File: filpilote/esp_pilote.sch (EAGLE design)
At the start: 22 parts, among them IC1 ACS758LCB-050B-PFF-T

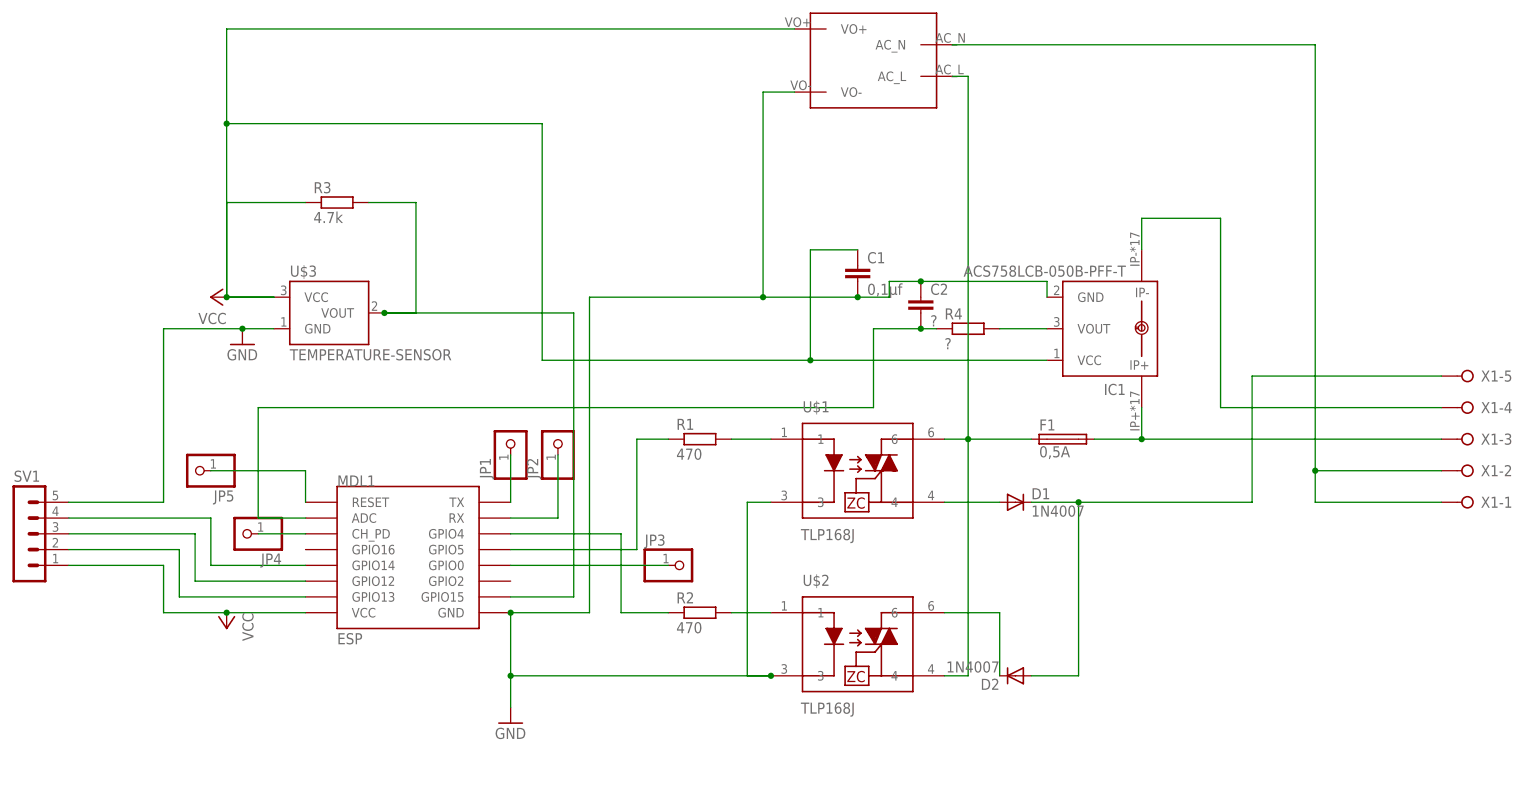
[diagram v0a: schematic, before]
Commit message: Mise à jour PCB
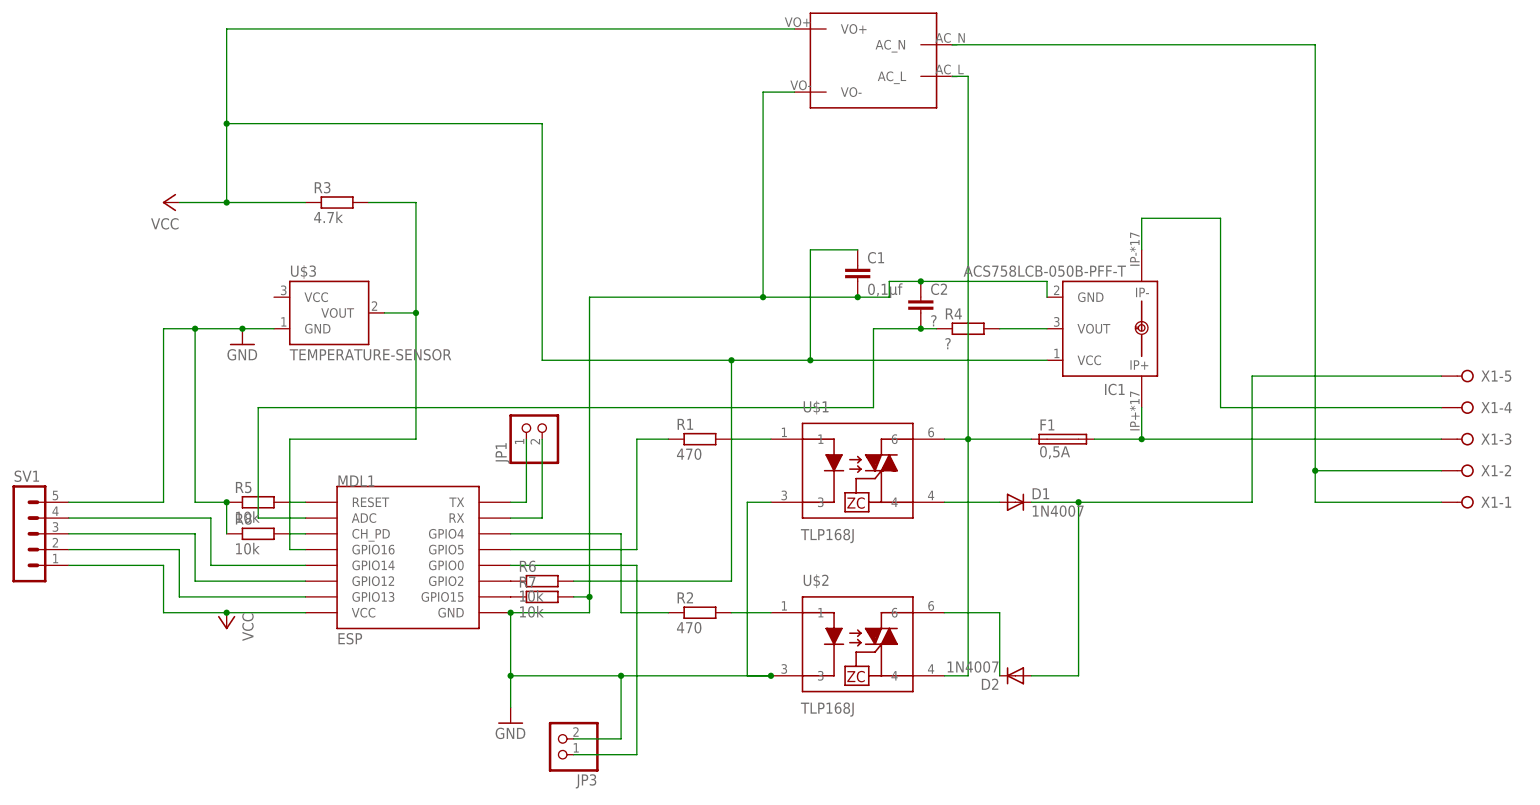
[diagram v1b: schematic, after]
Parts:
- removed JP2, JP4, JP5: (no value), pinhead:PINHD-1X1
- added R5, R6, R7, R8: 10k, rcl:R-EU_0204/7
- JP1, JP3: device pinhead:PINHD-1X1 -> pinhead:PINHD-1X2
- U$4: value HLK-PM03 -> MAINS_CONVERTERS
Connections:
- removed net VCC+3.3V: C1.1, IC1.VCC, MDL1.VCC, R3.1, SV1.1, U$3.VCC, U$4.VO+
- new net N$16: MDL1.CH_PD, R8.2
- new net N$18: MDL1.GPIO15, R7.1
- new net VCC: C1.1, IC1.VCC, MDL1.VCC, R3.1, R6.2, SV1.1, U$4.VO+
- net GND: now also JP3.2, R5.1, R7.2, R8.1
- net N$13: now also MDL1.RESET, R5.2; no longer JP4.1, MDL1.CH_PD
- net N$15: now also JP1.2; no longer JP2.1
- net N$17: now also MDL1.GPIO2, R6.1; no longer JP5.1, MDL1.RESET
- net N$9: now also MDL1.GPIO16; no longer MDL1.GPIO15
